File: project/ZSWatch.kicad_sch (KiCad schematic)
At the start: 32 parts, among them IC1 AT25SL128A, IC2 NX3DV42, IC3 nPM1300-QEXX, M1 NORA-B106, X1 VDISPLAY, X2 DOCK, X3 VBUS, X4 VBAT, X5 INT

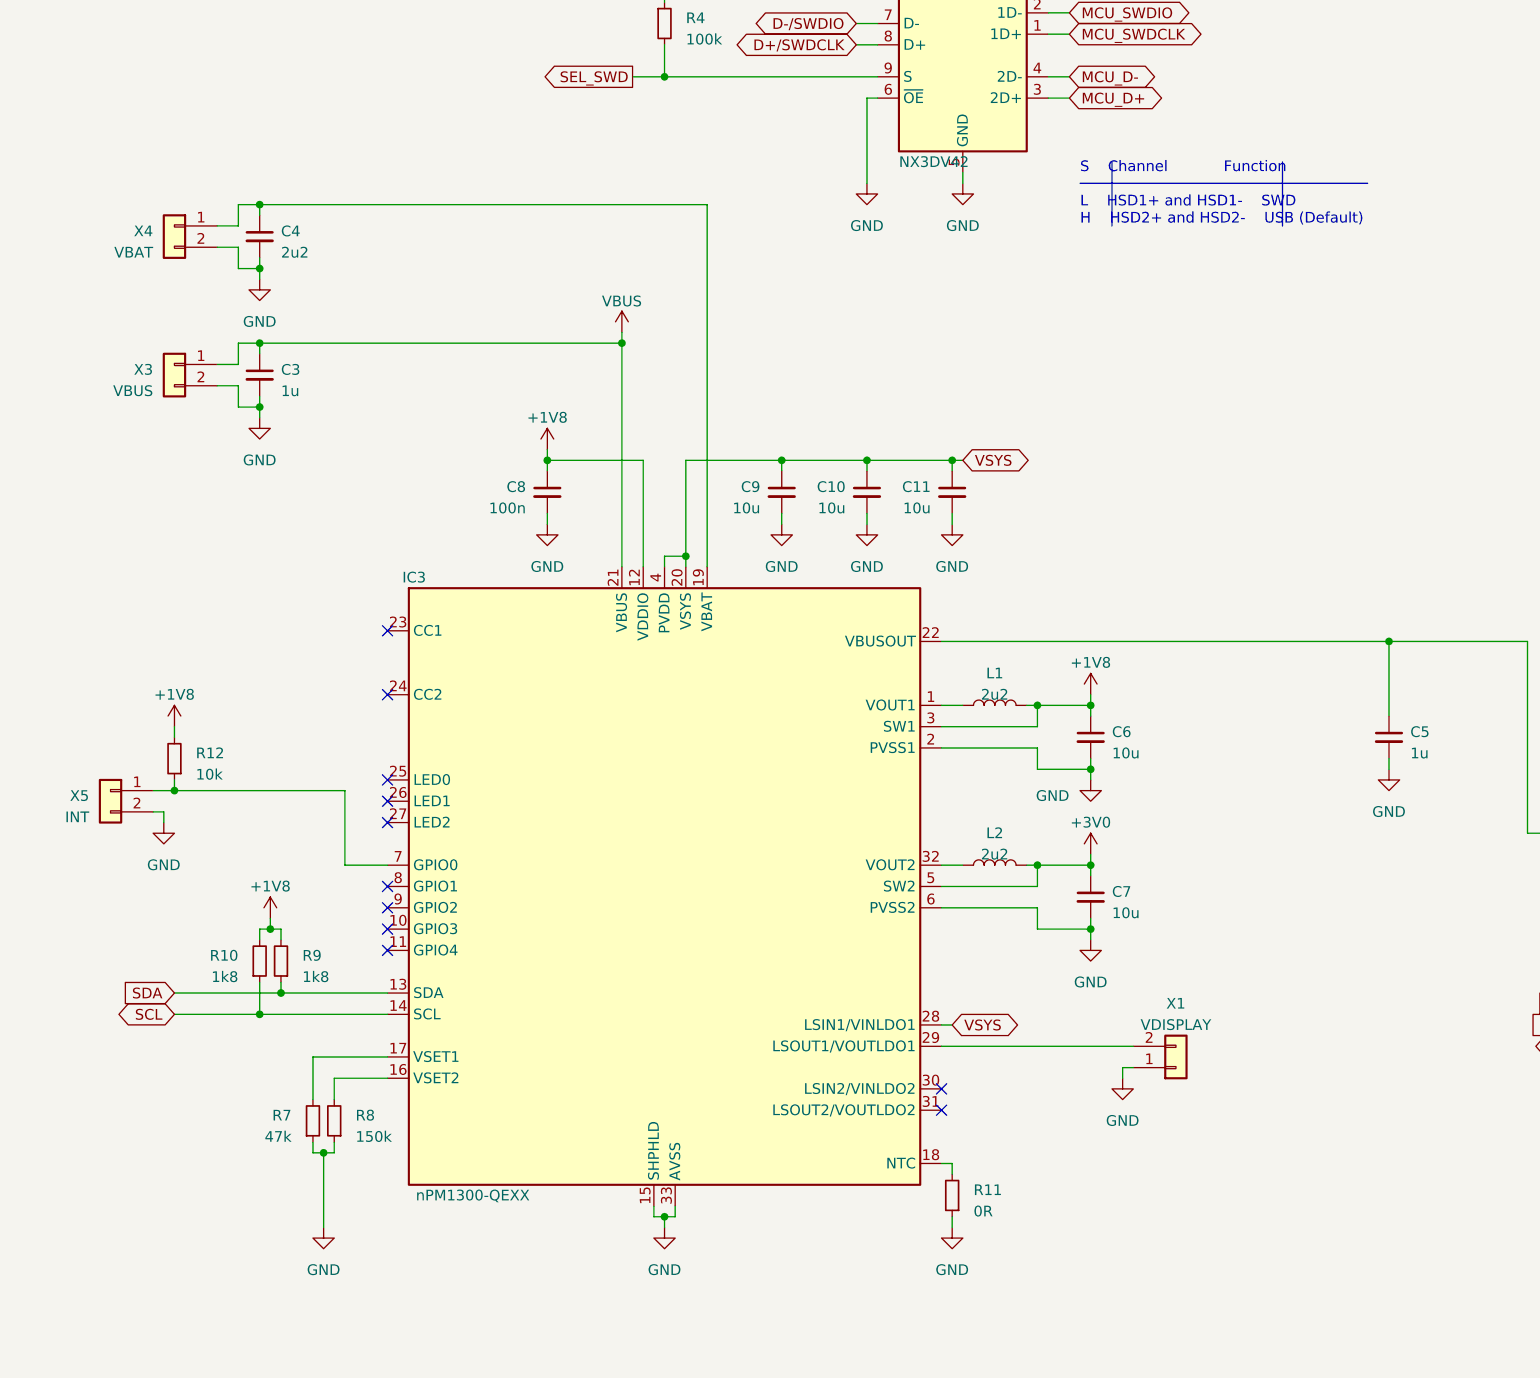
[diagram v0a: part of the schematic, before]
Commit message: Working on nPM1300 design
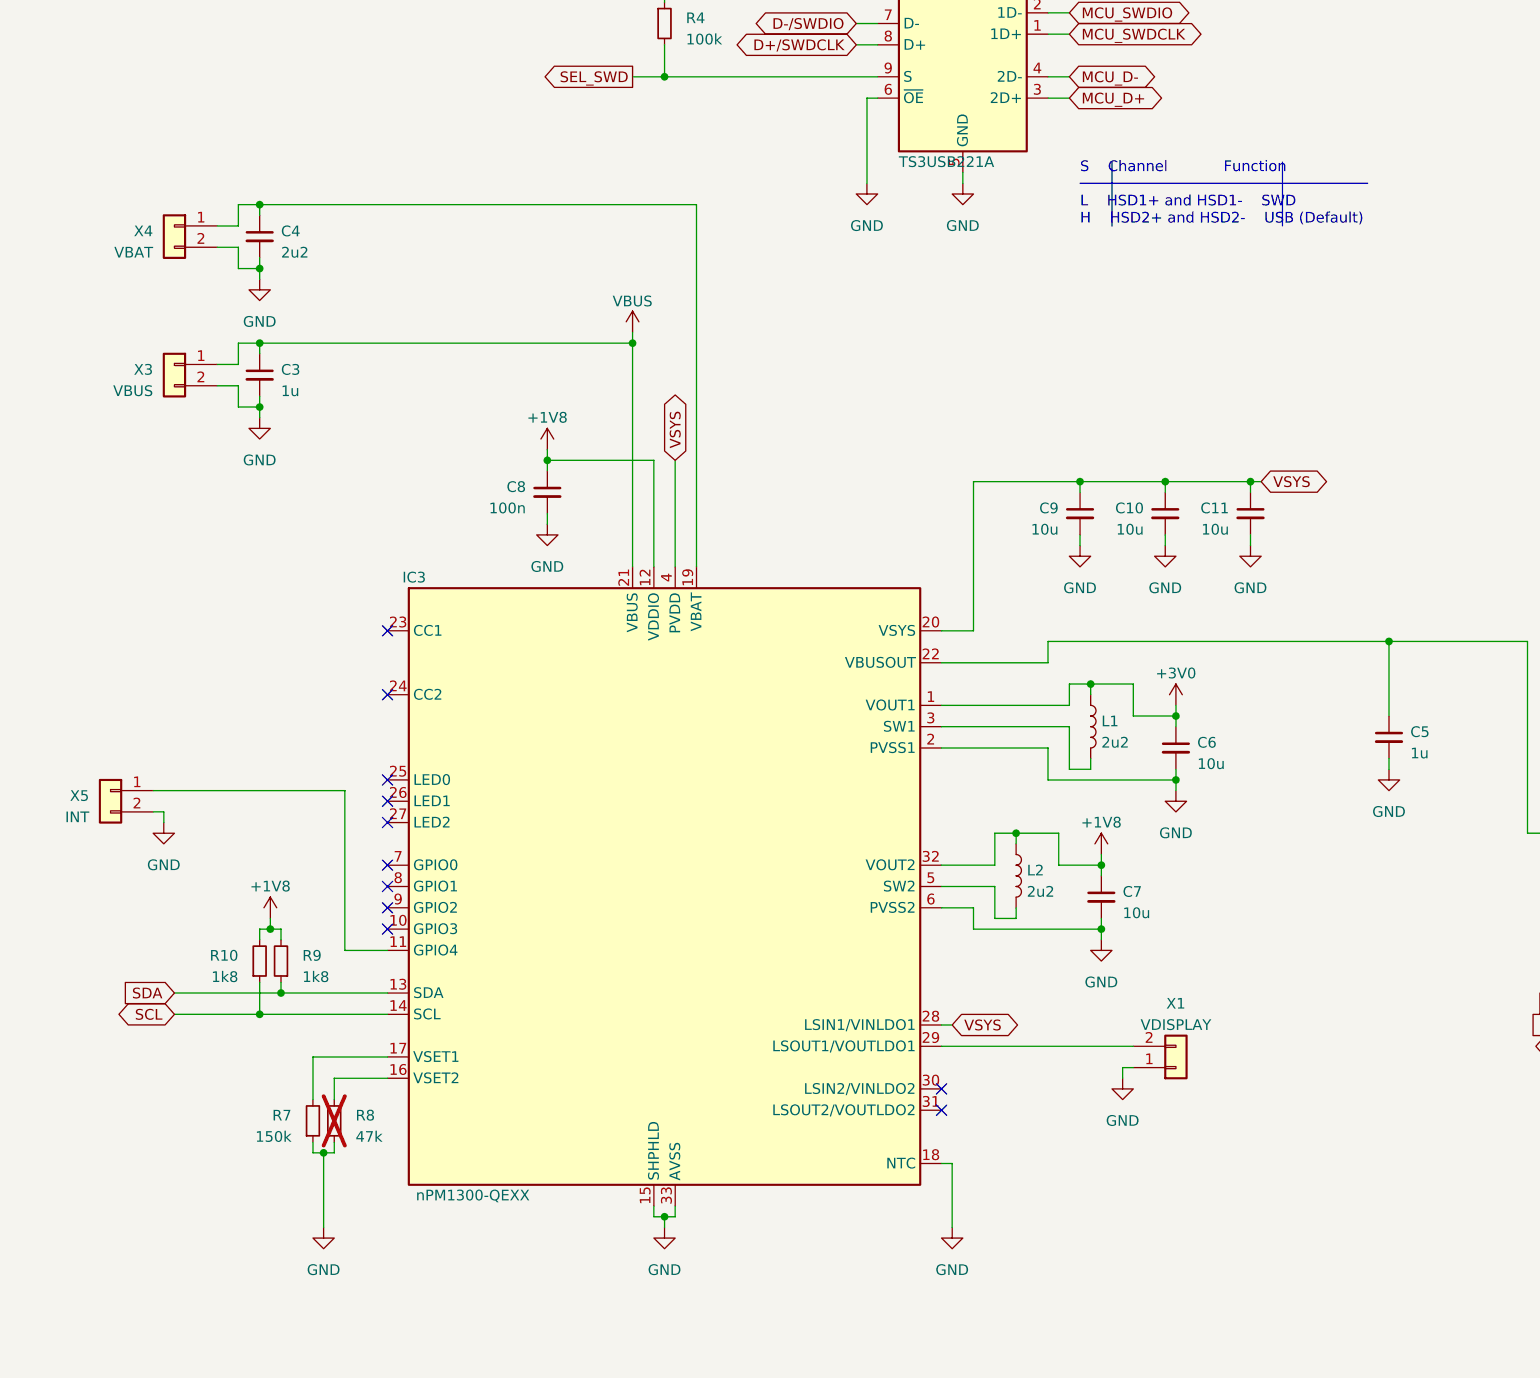
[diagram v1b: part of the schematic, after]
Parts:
- removed R11: 0R, Resistor_SMD:R_0603_1608Metric, symbol Device:R_Small
- removed R12: 10k, Resistor_SMD:R_0603_1608Metric, symbol Device:R_Small
- C10, C11, C6, C7, C9: Distributor (none) -> Mouser; Mfr. (none) -> KYOCERA AVX; Mfr. No. (none) -> CM105X5R106M25AT; Order Number (none) -> 346-CM105X5R106M25AT
- IC2: value NX3DV42 -> TS3USB221A; footprint (none) -> Package_QFN:UQFN-10_1.55x2.05mm_P0.5mm; Distributor (none) -> Mouser; Mfr. (none) -> Texas Instruments; Mfr. No. (none) -> TS3USB221A; Order Number (none) -> 595-TS3USB221A
- L1, L2: footprint (none) -> Inductor_SMD_Kampi:L_0806_2016; Distributor (none) -> Mouser; Mfr. (none) -> Samsung Electro-Mechanics; Mfr. No. (none) -> CIGT201610EH2R2MNE; Order Number (none) -> 187-CIGT201610EH2R2M
- R7: value 47k -> 150k
- R8: value 150k -> 47k; now not fitted; now left out of the parts list
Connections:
- net +1V8: now also C7.1, IC3.32 (VOUT2), L2.1; no longer C6.1, IC3.3 (SW1), L1.2
- net +3V0: now also C6.1, IC3.1 (VOUT1), L1.1; no longer C7.1, IC3.5 (SW2), L2.2
- net GND: now also IC3.18 (NTC)
- net at X5.1 (Pin_1): now also IC3.11 (GPIO4); no longer IC3.7 (GPIO0)
- new net: IC3.5 (SW2), L2.2
- new net: IC3.3 (SW1), L1.2
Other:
- moved on the sheet: C10, C11, C6, C7, C9, L1

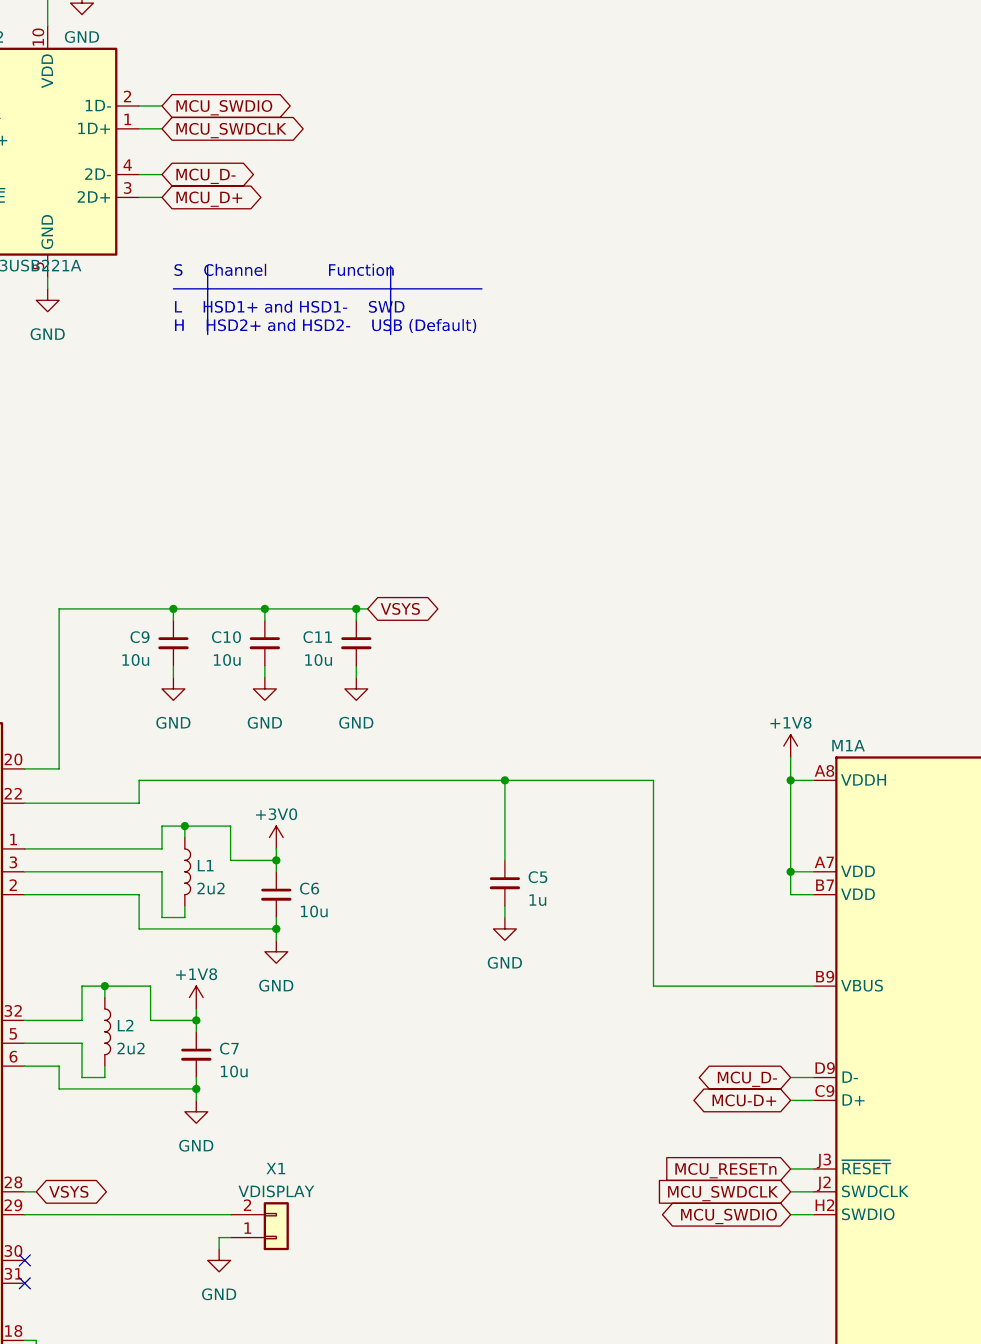
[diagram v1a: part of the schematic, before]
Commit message: Working on nPM1300 design
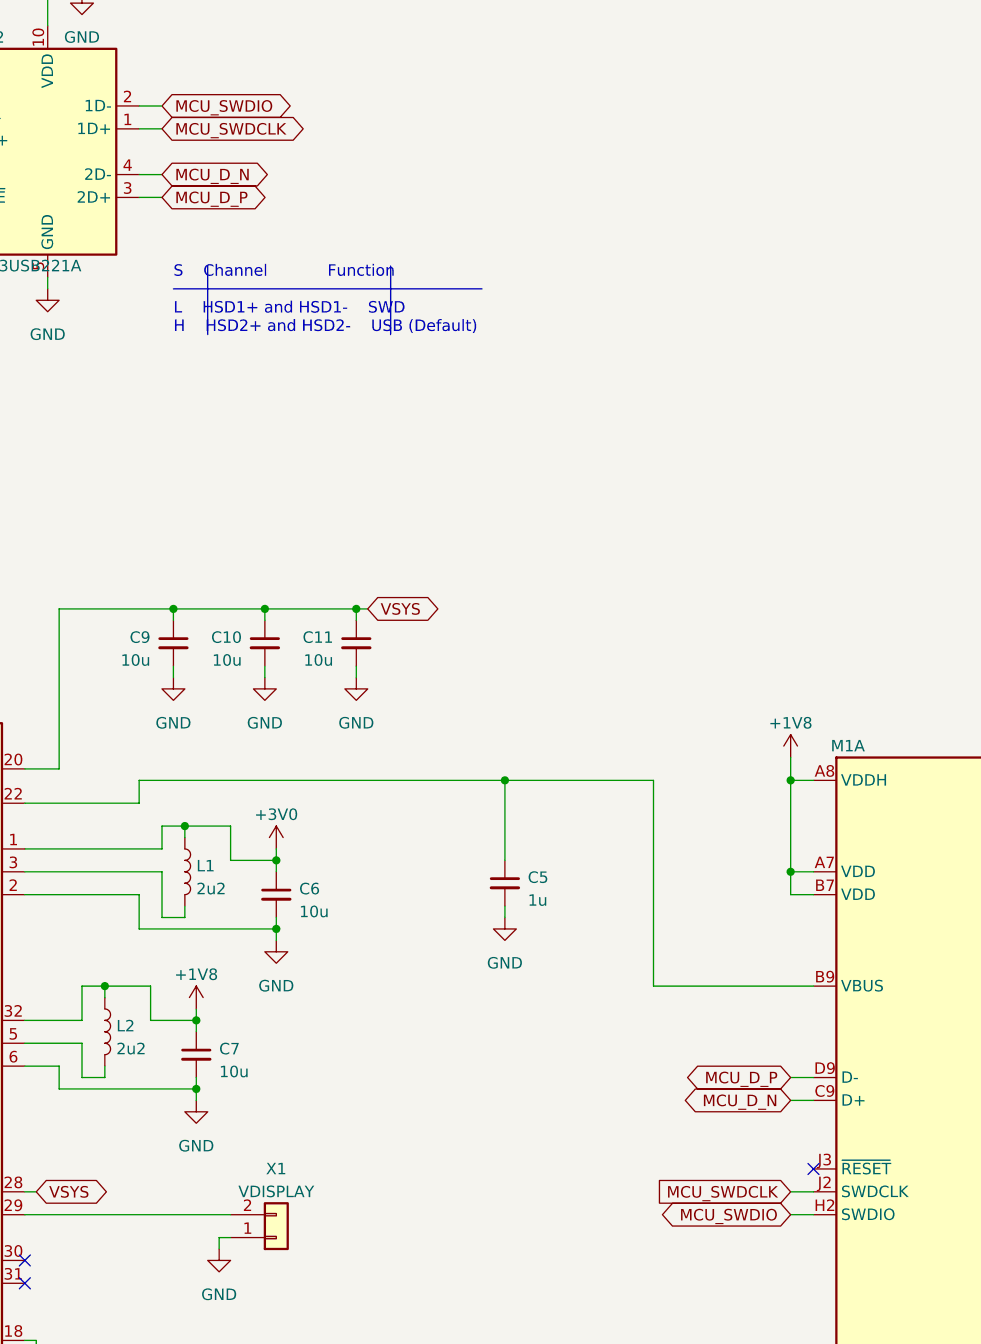
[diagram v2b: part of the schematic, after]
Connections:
- net MCU-D+ renamed MCU_D_N
- net MCU_D_N: now also IC2.4 (2D-)
- net MCU_D+ renamed MCU_D_P
- net MCU_D_P: now also M1.D9 (D-)
- removed net MCU_D-: IC2.4 (2D-), M1.D9 (D-)
- net MCU_RESETn: no longer names the net of M1.J3 (~{RESET})
- no-connect marks 60 -> 61
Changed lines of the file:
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@@
   (no_connect (at 367.03 154.94))
   (no_connect (at 55.88 151.13))
+  (no_connect (at 209.55 162.56))
   (no_connect (at 306.07 106.68))
   (no_connect (at 306.07 132.08))
@@
     (stroke (width 0) (type default))
   )
-  (wire (pts (xy 207.01 162.56) (xy 209.55 162.56))
-    (stroke (width 0) (type default))
-  )
   (wire (pts (xy 143.51 170.18) (xy 143.51 171.45))
     (stroke (width 0) (type default))
@@
     (effects (font (size 1.27 1.27)) (justify left bottom))
   )
-  (global_label "MCU_RESETn" (shape input) (at 207.01 162.56 180) (fields_autoplaced)
-    (effects (font (size 1.27 1.27)) (justify right))
-    (property "Intersheetrefs" "${INTERSHEET_REFS}" (at 192.1906 162.56 0)
-      (effects (font (size 1.27 1.27)) (justify right) hide)
-    )
-  )
   (global_label "SEL_SWD" (shape output) (at 27.94 21.59 0) (fields_autoplaced)
     (effects (font (size 1.27 1.27)) (justify left))
@@
     )
   )
-  (global_label "MCU_D-" (shape bidirectional) (at 137.16 52.07 0) (fields_autoplaced)
-    (effects (font (size 1.27 1.27)) (justify left))
-    (property "Intersheetrefs" "${INTERSHEET_REFS}" (at 149.039 52.07 0)
+  (global_label "MCU_D_N" (shape bidirectional) (at 137.16 52.07 0) (fields_autoplaced)
+    (effects (font (size 1.27 1.27)) (justify left))
+    (property "Intersheetrefs" "${INTERSHEET_REFS}" (at 149.7647 52.07 0)
       (effects (font (size 1.27 1.27)) (justify left) hide)
     )
@@
     )
   )
-  (global_label "MCU_D+" (shape bidirectional) (at 137.16 54.61 0) (fields_autoplaced)
-    (effects (font (size 1.27 1.27)) (justify left))
-    (property "Intersheetrefs" "${INTERSHEET_REFS}" (at 149.039 54.61 0)
+  (global_label "MCU_D_P" (shape bidirectional) (at 137.16 54.61 0) (fields_autoplaced)
+    (effects (font (size 1.27 1.27)) (justify left))
+    (property "Intersheetrefs" "${INTERSHEET_REFS}" (at 149.7042 54.61 0)
       (effects (font (size 1.27 1.27)) (justify left) hide)
     )
@@
     )
   )
-  (global_label "MCU_D-" (shape bidirectional) (at 207.01 152.4 180) (fields_autoplaced)
-    (effects (font (size 1.27 1.27)) (justify right))
-    (property "Intersheetrefs" "${INTERSHEET_REFS}" (at 195.131 152.4 0)
+  (global_label "MCU_D_P" (shape bidirectional) (at 207.01 152.4 180) (fields_autoplaced)
+    (effects (font (size 1.27 1.27)) (justify right))
+    (property "Intersheetrefs" "${INTERSHEET_REFS}" (at 194.4658 152.4 0)
       (effects (font (size 1.27 1.27)) (justify right) hide)
     )
@@
     )
   )
-  (global_label "MCU-D+" (shape bidirectional) (at 207.01 154.94 180) (fields_autoplaced)
-    (effects (font (size 1.27 1.27)) (justify right))
-    (property "Intersheetrefs" "${INTERSHEET_REFS}" (at 194.5262 154.94 0)
-      (effects (font (size 1.27 1.27)) (justify right) hide)
-    )
+  (global_label "MCU_D_N" (shape bidirectional) (at 207.01 154.94 180) (fields_autoplaced)
+    (effects (font (size 1.27 1.27)) (justify right))
+    (property "Intersheetrefs" "${INTERSHEET_REFS}" (at 194.4053 154.94 0)
+      (effects (font (size 1.27 1.27)) (justify right) hide)
+    )
